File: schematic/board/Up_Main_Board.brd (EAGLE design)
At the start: 79.9 x 73.5 mm, 18 parts

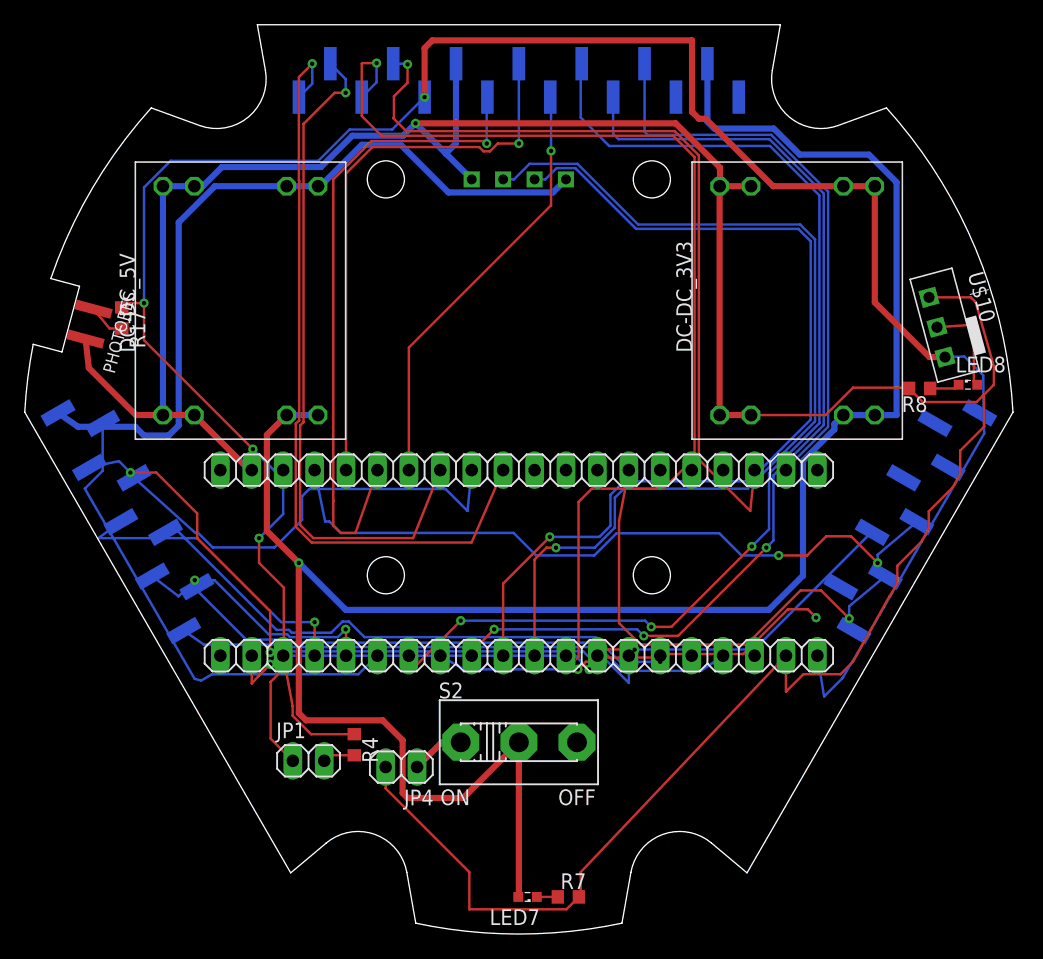
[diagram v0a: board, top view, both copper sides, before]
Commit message: поправил контур всех плат
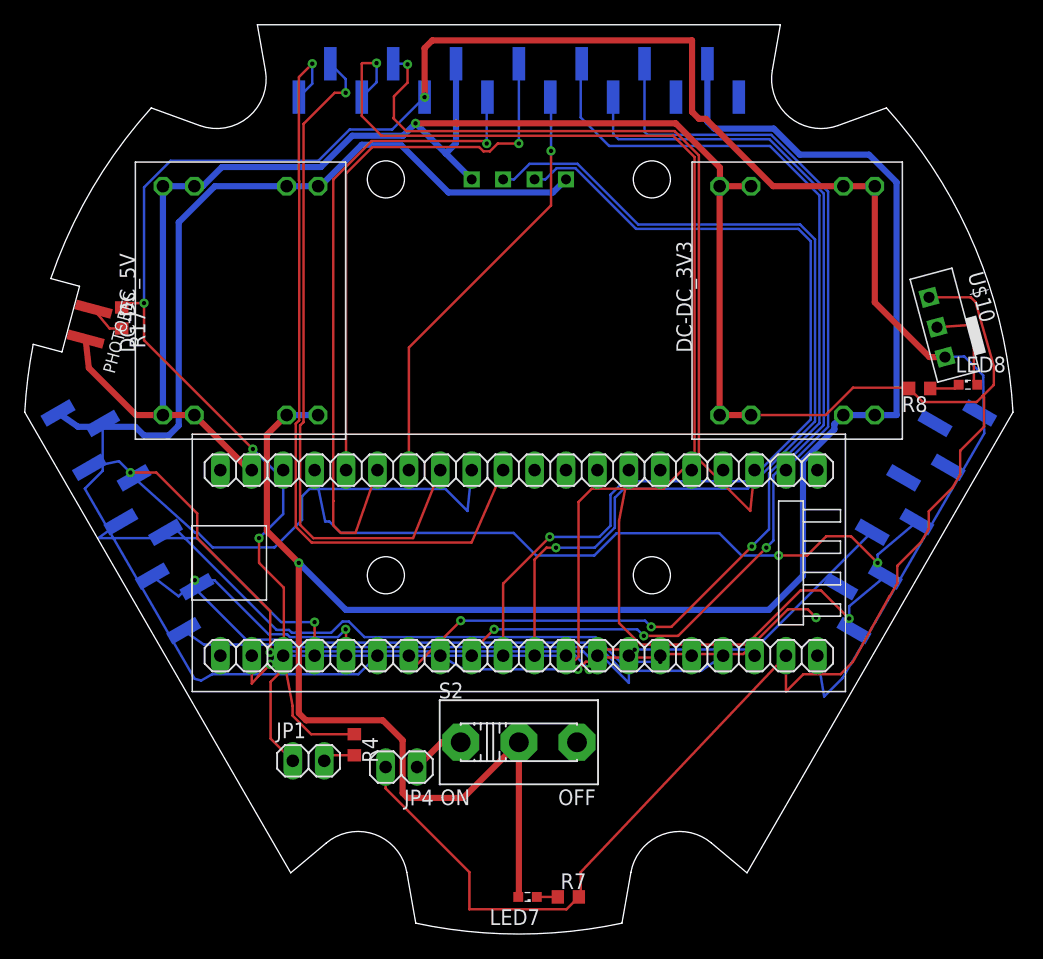
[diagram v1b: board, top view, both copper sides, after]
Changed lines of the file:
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@@
 <wire x1="13.06603125" y1="57.04941875" x2="14.48953125" y2="62.362009375" width="0.001" layer="20"/>
 <wire x1="31.55733125" y1="14.94365" x2="10.0594" y2="52.179140625" width="0.001" layer="20"/>
-<wire x1="79.71443125" y1="76.777840625" x2="75.794009375" y2="75.35091875" width="0.001" layer="20"/>
+<wire x1="79.71443125" y1="76.777840625" x2="75.794" y2="75.3509" width="0.001" layer="20"/>
 <wire x1="28.86165" y1="83.5" x2="29.5133" y2="79.80428125" width="0.001" layer="20"/>
 <wire x1="40.94246875" y1="14.98626875" x2="41.66693125" y2="10.87763125" width="0.001" layer="20"/>
 <wire x1="65.56791875" y1="17.355859375" x2="68.44266875" y2="14.94365" width="0.001" layer="20"/>
 <wire x1="10.74263125" y1="57.67196875" x2="13.06603125" y2="57.04941875" width="0.001" layer="20"/>
-<wire x1="14.48953125" y1="62.362009375" x2="12.166140625" y2="62.984559375" width="0.001" layer="20"/>
+<wire x1="14.48953125" y1="62.362009375" x2="12.1661" y2="62.984" width="0.001" layer="20"/>
 <wire x1="71.13835" y1="83.5" x2="70.4867" y2="79.80428125" width="0.001" layer="20"/>
 <wire x1="58.33306875" y1="10.87763125" x2="59.05753125" y2="14.98626875" width="0.001" layer="20"/>
@@
 <wire x1="89.9406" y1="52.179140625" x2="68.44266875" y2="14.94365" width="0.001" layer="20"/>
 <wire x1="28.86165" y1="83.5" x2="71.13835" y2="83.5" width="0.001" layer="20"/>
-<wire x1="20.28556875" y1="76.777840625" x2="12.166134375" y2="62.9845625" width="0.001" layer="20" curve="23.082126"/>
+<wire x1="20.28556875" y1="76.777840625" x2="12.1661" y2="62.984" width="0.001" layer="20" curve="23.082126"/>
 <wire x1="10.74263125" y1="57.67196875" x2="10.0594" y2="52.179140625" width="0.001" layer="20" curve="7.934868"/>
 <wire x1="41.66693125" y1="10.87763125" x2="58.33306875" y2="10.87763125" width="0.001" layer="20" curve="24.048625"/>
 <wire x1="89.9406" y1="52.179140625" x2="79.71443125" y2="76.777840625" width="0.001" layer="20" curve="38.901385"/>
 <wire x1="40.94246875" y1="14.98626875" x2="34.43208125" y2="17.355859375" width="0.001" layer="20" curve="120.000035"/>
-<wire x1="65.56791875" y1="17.355859375" x2="59.057534375" y2="14.98626875" width="0.001" layer="20" curve="120.000001"/>
-<wire x1="70.4867" y1="79.80428125" x2="75.79400625" y2="75.350921875" width="0.001" layer="20" curve="120.000013"/>
-<wire x1="24.205990625" y1="75.35091875" x2="29.513296875" y2="79.80428125" width="0.001" layer="20" curve="119.999997"/>
+<wire x1="65.56791875" y1="17.355859375" x2="59.05753125" y2="14.98626875" width="0.001" layer="20" curve="120.000001"/>
+<wire x1="70.4867" y1="79.80428125" x2="75.794" y2="75.3509" width="0.001" layer="20" curve="120.000013"/>
+<wire x1="24.205990625" y1="75.35091875" x2="29.5133" y2="79.80428125" width="0.001" layer="20" curve="119.999997"/>
 </plain>
 <attributes>
